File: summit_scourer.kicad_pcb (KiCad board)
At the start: 4 copper layers, 78 x 47 mm, 117 parts, among them J2 Conn_Coaxial, J3 PTT/Mic, J4 Headphone, J5 Internal_SPK, J7 Prog, J8 Conn_01x06_Socket, Q1 BS170, Q2 2N7002H, Q3 BS170, Q4 BS170, SW7 Key, SW8 RotaryEncoder, U1 SI4732-A10-GS, U3 Si5351A-B-GT, U4 ESP32-WROOM-32UE, U5 AZ1117-3.3, U6 LM4808MX_NOPB, U7 AZ1117-3.3, U8 74AC00, Y1 32.768 KHz, Y3 25MHz

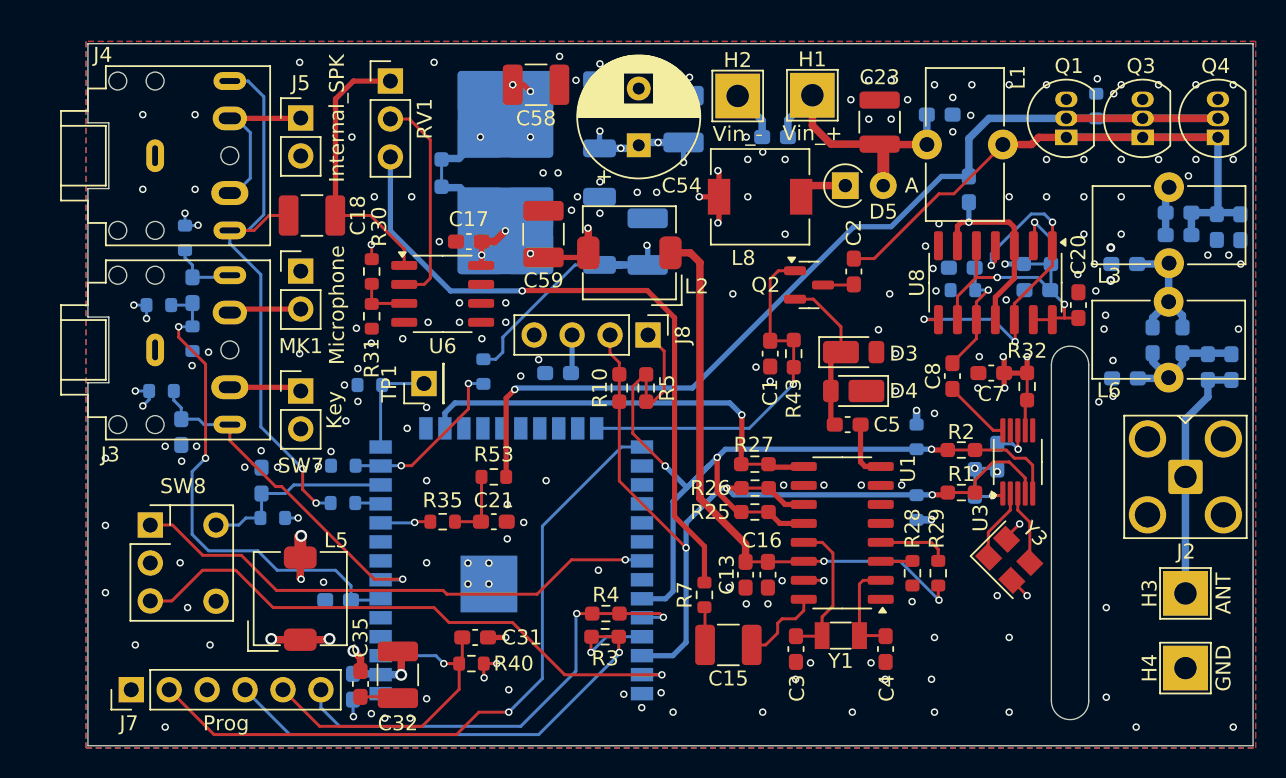
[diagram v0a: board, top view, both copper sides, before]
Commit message: Add files via upload
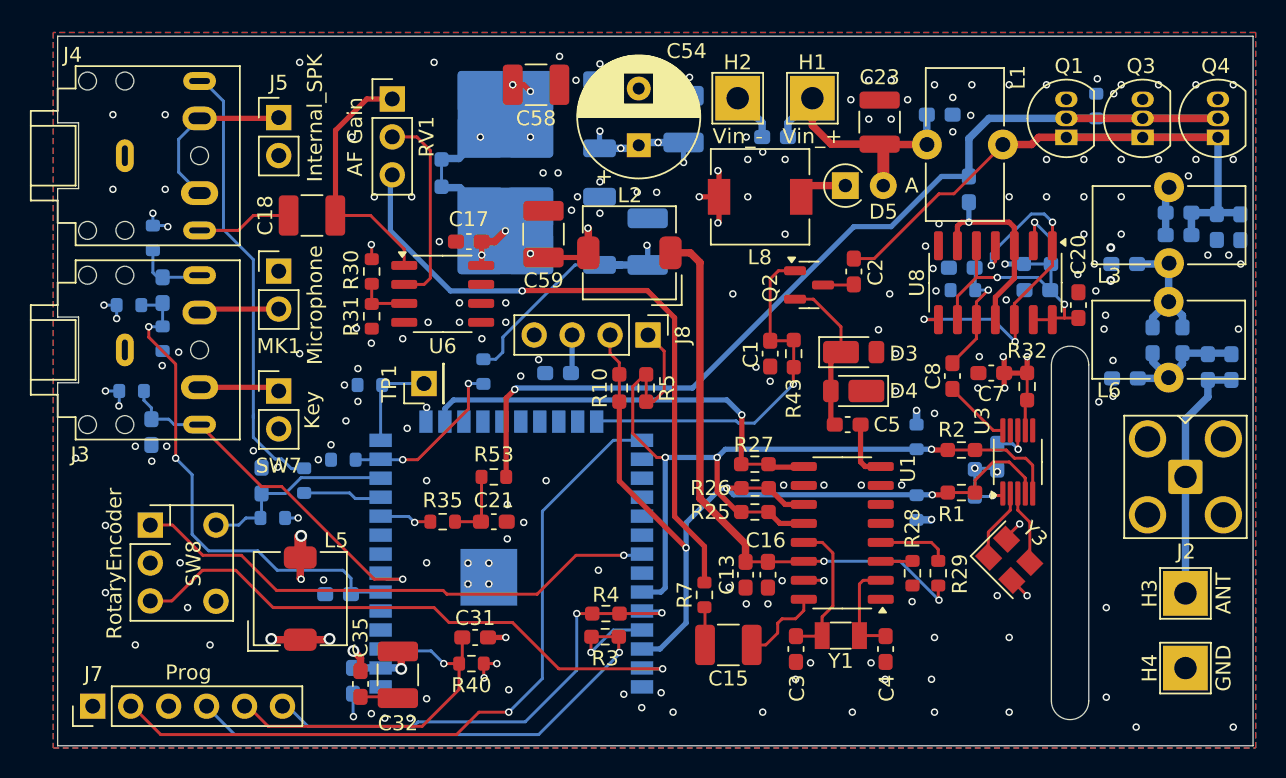
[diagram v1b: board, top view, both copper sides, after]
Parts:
- moved R49 3.00 mm to (122.8, 104.0), turned to 90 degrees
- moved J7 2.80 mm to (108.7, 119.1)
- moved R41 2.15 mm to (112.7, 87.8)
- moved J3 2.03 mm to (110.8, 95.2)
- moved J4 2.03 mm to (110.8, 82.2)
- moved C34 2.00 mm to (112.6, 100.8)
- moved C42 2.00 mm to (113.3, 91.2)
- moved R42 2.00 mm to (111.2, 98.0)
- moved R45 2.00 mm to (111.1, 92.2)
- moved R8 2.00 mm to (113.3, 94.5)
- moved J5 1.48 mm to (121.1, 79.7)
- moved MK1 1.48 mm to (121.1, 90.0)
- moved SW7 1.48 mm to (121.1, 98.0)
- moved RV1 1.21 mm to (128.7, 78.5)
- moved U4 0.45 mm to (136.7, 109.4)
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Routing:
- net /side_tone: track 1.78 -> 5.31 mm
- net /I2C_SDIO: track 44.2 -> 41.2 mm
- net /ESP_boot: track 46.8 -> 49.7 mm
- net /ESP_reset: track 22.9 -> 25.2 mm
- net /ESP_TX: track 29.7 -> 31.8 mm
- net Net-(U6-OUT_A): track 18.6 -> 17.0 mm
- net /ESP_RX: track 25.2 -> 26.6 mm
- net /PTT_key: track 23.5 -> 24.8 mm
- net Net-(R7-Pad2): track 45.0 -> 43.8 mm
- net Net-(U6-IN_A-): track 14.4 -> 13.4 mm
- net /I2C_SCL: track 42.7 -> 41.7 mm
- net /onboard_mic: track 4.85 -> 5.40 mm
- net /onboard_key: track 4.85 -> 5.40 mm
- net GND: track 15.3 -> 15.6 mm, vias 179 -> 177
- net /audio_out_right: track 39.3 -> 39.5 mm, vias 2 -> 0
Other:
- board size 78 x 47 mm -> 80 x 47.5 mm
- board text added: "AF Gain"
